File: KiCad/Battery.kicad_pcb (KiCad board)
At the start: 2 copper layers, 19 x 29 mm, 26 parts, among them J1 Connector, J2 USB-C, J3 DC, Q1 RN1701, U1 ESP32-WROOM-32, U2 FT231XQ, U3 NX6020CAKS

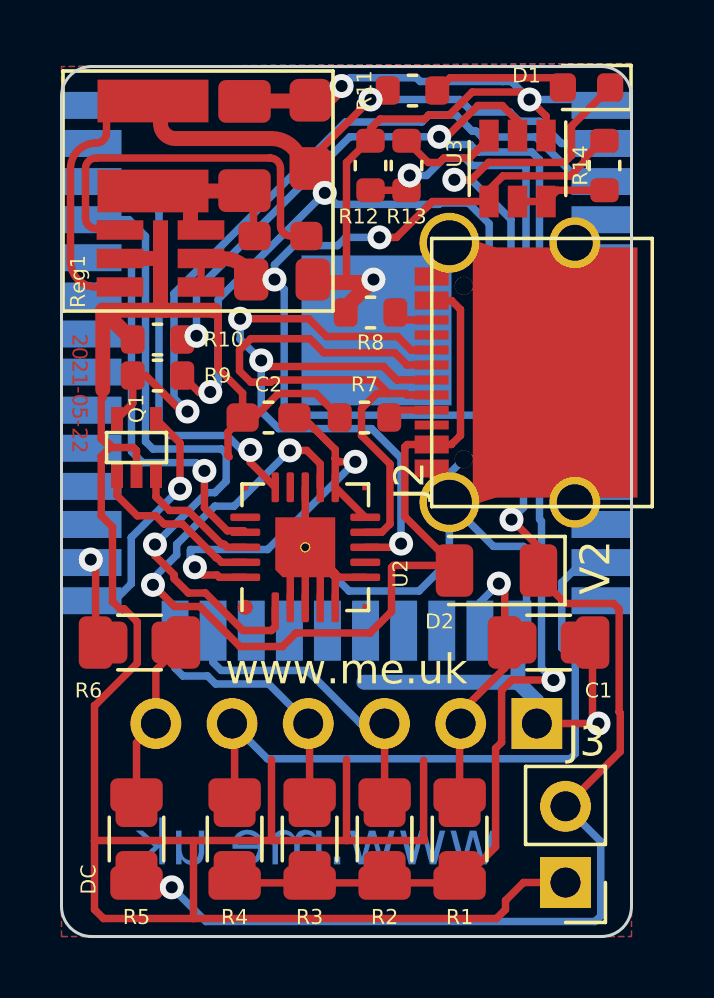
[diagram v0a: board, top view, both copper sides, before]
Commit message: Tweak
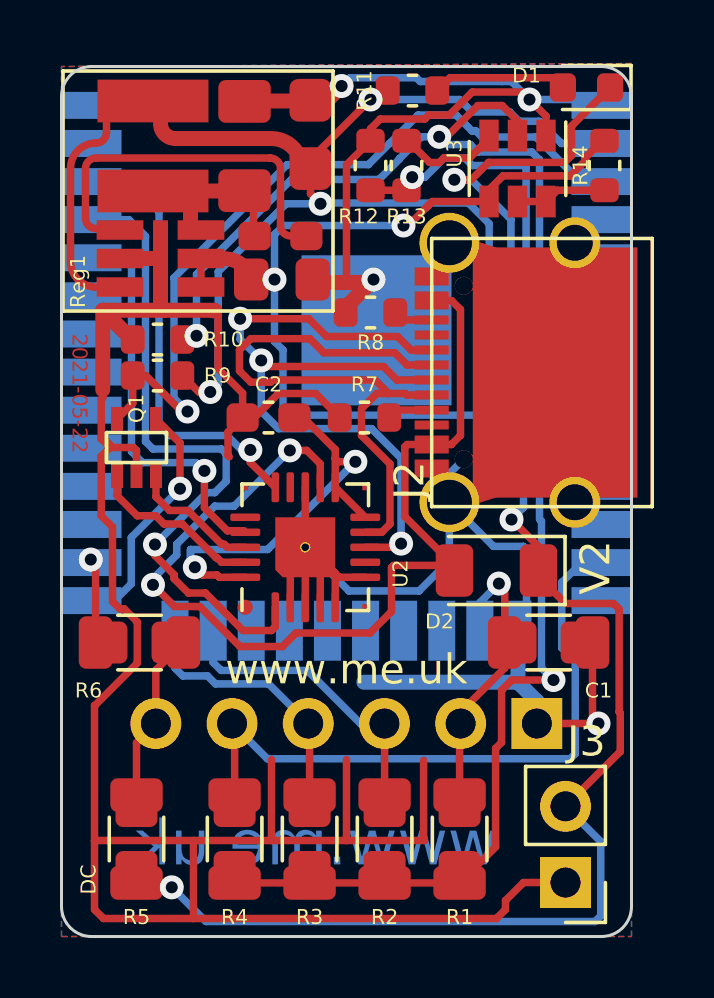
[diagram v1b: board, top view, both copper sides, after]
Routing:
- net DC: track 65.4 -> 66.2 mm
